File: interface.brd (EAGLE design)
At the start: 70 x 100 mm, 78 parts, among them CN1 61083-103400LF, CN2 61083-103400LF, CN3 FH52E-60S-0.5SH, CN4 2.1mm DC Jack, CN5 61 PIN 0.2mm FFC, Q1 2N7002, U1 TLV3201, U2 PI4ULS3V204ZBEX, U3 ADJ BUCK, U4 ADJ BUCK, U5 LM2731X, U6 TPS54233D

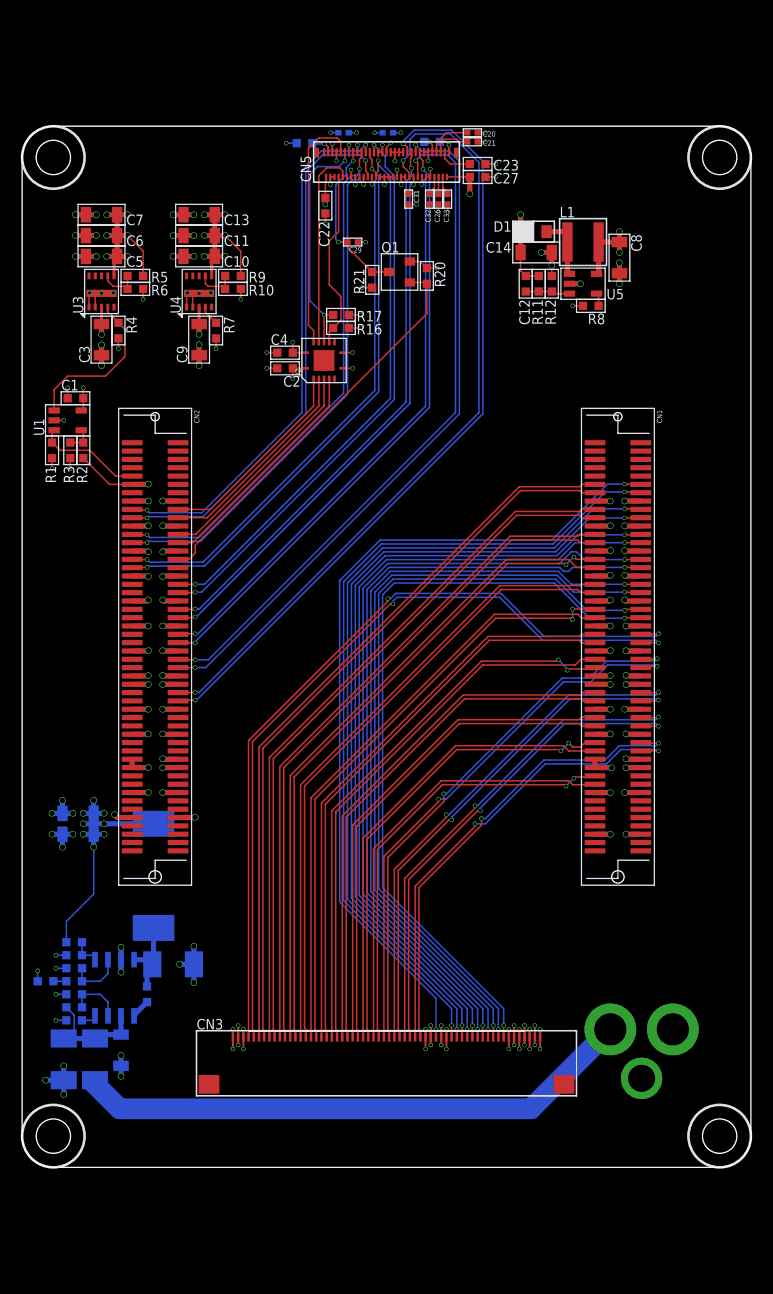
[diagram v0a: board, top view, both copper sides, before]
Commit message: Interface modified with in stock components
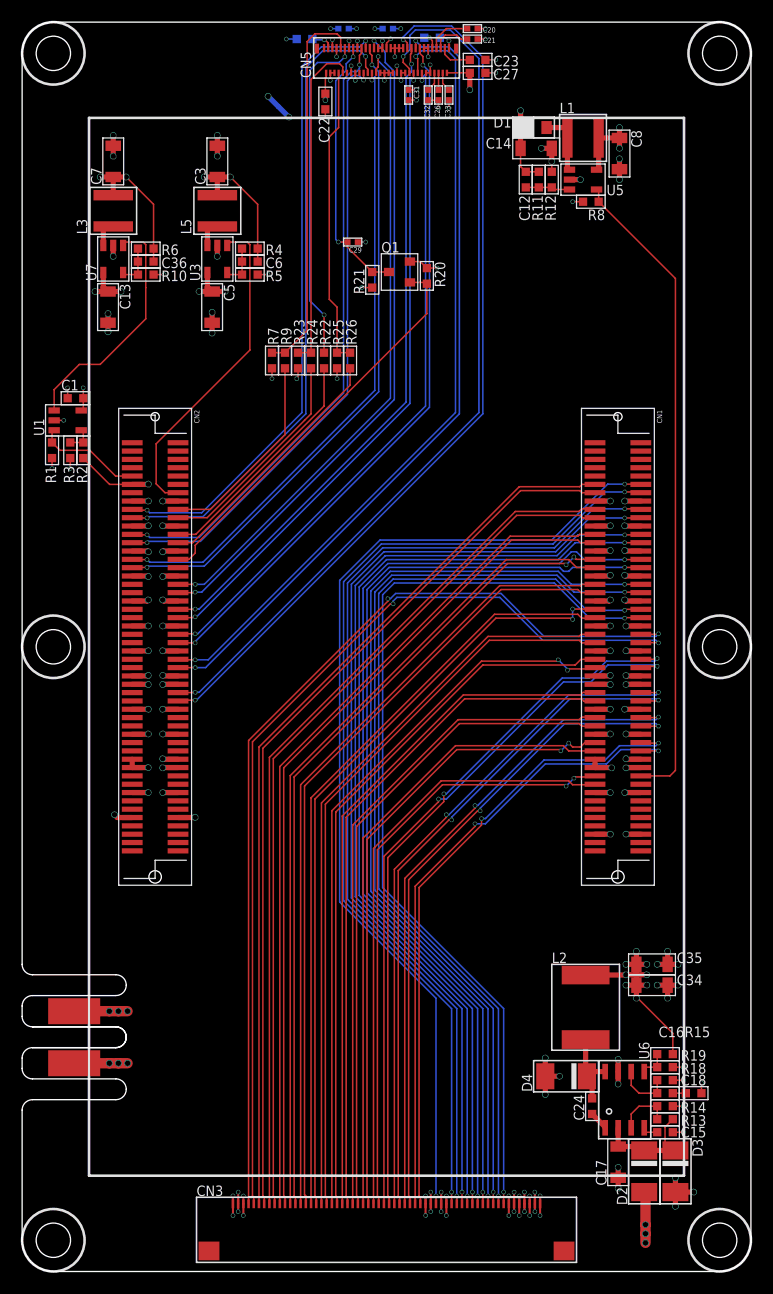
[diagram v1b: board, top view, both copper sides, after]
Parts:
- removed C10, C11: 22uF 6.3V, c_1206:1206
- removed C2, C4: 0.1uF 16V, c_0603:0603
- removed C9: 10uF 10V, c_1206:1206
- removed R16, R17: 10k, r_0603:0603
- removed U2: PI4ULS3V204ZBEX, ICs:TQFN14
- removed U4: ADJ BUCK, ICs:TI_MICROSIP_10
- added C36: 100pF 25V, c_0603:0603
- added CN6: PCB Tab, CONNECTORs:PCB_TAB_SMALL
- added L3, L5: 2.2uH 3A, INDUCTORS:IFSC-1515AH-01
- added MECH5, MECH6: 6mm x 3mm, MISC:MOUNTHOLE_6X3
- added R22: 10R, r_0603:0603
- added R23, R25: 1.5k, r_0603:0603
- added R24, R26: 680R, r_0603:0603
- added U7: PAM2312, ICs:SOT23-5
- C13, C5, C7: value 22uF 6.3V -> 10uF 10V
- C6: value 22uF 6.3V -> 100pF 25V; device c_1206:1206 -> c_0603:0603
- CN4: value 2.1mm DC Jack -> PCB Tab; device CONNECTORs:PJ-202AH -> CONNECTORs:PCB_TAB_SMALL
- L2: device INDUCTORS:MSS1038-223MLC -> INDUCTORS:ECS-MPIL0630
- R10: value 15k -> 150k
- R4: value 10k -> 200k
- R5: value 15k -> 100k
- R6: value 10k -> 475k
- R7: value 10k -> 1.5k
- R9: value 12.1k -> 680R
- U3: value ADJ BUCK -> PAM2312; device ICs:TI_MICROSIP_10 -> ICs:SOT23-5
- moved R15 63.2 mm to (29.5, -42.9), flipped to the top
- moved D3 59.7 mm to (27.8, -50.4), flipped to the top
- moved C15 57.8 mm to (26.8, -46.6), flipped to the top
- moved C16 57.8 mm to (26.8, -42.9), flipped to the top
- moved C18 57.8 mm to (26.8, -41.6), flipped to the top
- moved R13 57.8 mm to (26.8, -45.4), flipped to the top
- moved R14 57.8 mm to (26.8, -44.1), flipped to the top
- moved R18 57.8 mm to (26.8, -40.4), flipped to the top
- moved R19 57.8 mm to (26.8, -39.1), flipped to the top
- moved C34 57.0 mm to (25.5, -32.5), flipped to the top
- moved C35 57.0 mm to (25.5, -30.5), flipped to the top
- moved CN4 54.5 mm to (-30.0, -35.0), flipped to the top, turned to 90 degrees
- moved D2 53.8 mm to (24.8, -50.4), flipped to the top
- moved U6 50.2 mm to (22.9, -43.5), flipped to the top
- moved C17 48.9 mm to (22.2, -49.5), flipped to the top
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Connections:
- removed net N$1: R10.2, R9.1, U4.7
- removed net N$36: CN1.81
- removed net N$67: R5.1, R6.2, U3.7
- removed net N$79: CN2.13
- new net N$14: L3.1, U7.3
- new net N$15: C36.1, R10.2, R6.1, U7.5
- new net N$17: L5.1, U3.3
- new net N$18: C6.1, R4.1, R5.2, U3.5
- net EVF_PWR_10V_EN: now also CN1.81
- net EVF_PWR_1V8: now also C3.2, C6.2, L5.2, R4.2; no longer C10.2, C11.2, C13.2, C4.1, R16.2, R9.2, U2.14, U4.6
- net EVF_PWR_1V8_EN: now also CN2.13, U3.1; no longer R7.2, U4.4
- net EVF_SPI_!CS: now also R25.2, R26.2; no longer R16.1, U2.10
- net EVF_SPI_MISO: now also R22.2; no longer R17.1, U2.11
- net EVF_SPI_MOSI: now also R23.2, R24.2; no longer U2.12
- net EVF_SPI_SCLK: now also R7.2, R9.2; no longer U2.13
- net FPGA_EVF_SPI_!CS: now also R26.1; no longer U2.5
- net FPGA_EVF_SPI_MISO: now also R22.1; no longer U2.4
- net FPGA_EVF_SPI_MOSI: now also R24.1; no longer U2.3
- net FPGA_EVF_SPI_SCLK: now also R9.1; no longer U2.2
- net GND: now also CN6.1, R23.1, R25.1, R5.1, U7.2; no longer C10.1, C11.1, C2.2, C4.2, C6.1, C9.1, CN4.2, R17.2, R4.1, R6.1, U2.7, U3.1, U3.PAD, U4.1, U4.2, U4.PAD
- net SYS_PWR_2V5: now also C36.2, L3.2, R6.2; no longer C2.1, C5.2, C6.2, R5.2, U2.1, U2.8, U3.6
- net SYS_PWR_5V: now also C13.2, C5.2, U3.4, U7.4; no longer C3.2, C9.2, U3.3, U4.3
- net SYS_VCCO_EN: now also U7.1; no longer R4.2, U3.4
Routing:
- net EVF_PWR_10V_EN: track 1.26 -> 62.5 mm
- net EVF_PWR_1V8_EN: track 1.92 -> 31.6 mm
- net EVF_PWR_1V8: track 111.6 -> 89.5 mm, vias 18 -> 12
- net N$12: track 54.1 -> 72.7 mm, vias 0 -> 6
- net EVF_PWR_10V: track 73.8 -> 57.2 mm, vias 3 -> 5
- net SEN_PWR_EN: track 80.5 -> 96.5 mm
- net SEN_T_D6_N: track 53.1 -> 69.1 mm
- net SEN_T_D15_P: track 68.1 -> 84.1 mm
- net SEN_TEXP0: track 76.1 -> 92.1 mm
- net SEN_TDIG0: track 74.4 -> 90.4 mm
- net SEN_B_D6_P: track 50.4 -> 66.4 mm
- net SEN_B_D12_N: track 53.6 -> 69.6 mm
- net SEN_T_D9_N: track 55.7 -> 71.7 mm
- net SEN_T_D0_P: track 45.3 -> 61.3 mm
- net SEN_B_D9_P: track 48.0 -> 64.0 mm
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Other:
- board size 70 x 100 mm -> 70 x 120 mm
